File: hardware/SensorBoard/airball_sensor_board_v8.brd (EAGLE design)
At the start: 5.6 x 9.2 mm, 61 parts, among them IC1 CP2102, J2 USB Female Type C Connector, T1 BC846, T2 BC846, U1 BQ24075, U2 BQ27441-G1, U3 BMP388, U4 ESP-WROOM-32, U7 SP0503BAHT

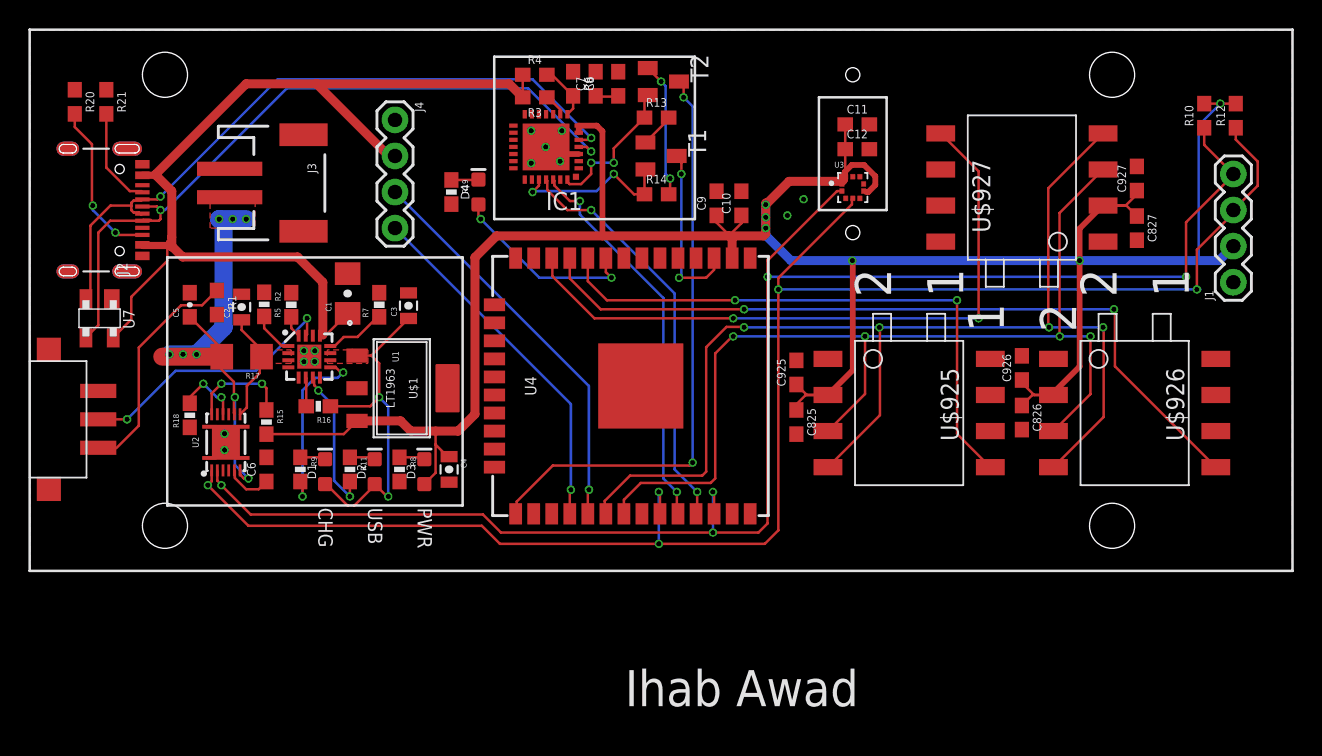
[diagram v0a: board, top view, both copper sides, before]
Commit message: Finishing touches to the board, sent to manufacturing.
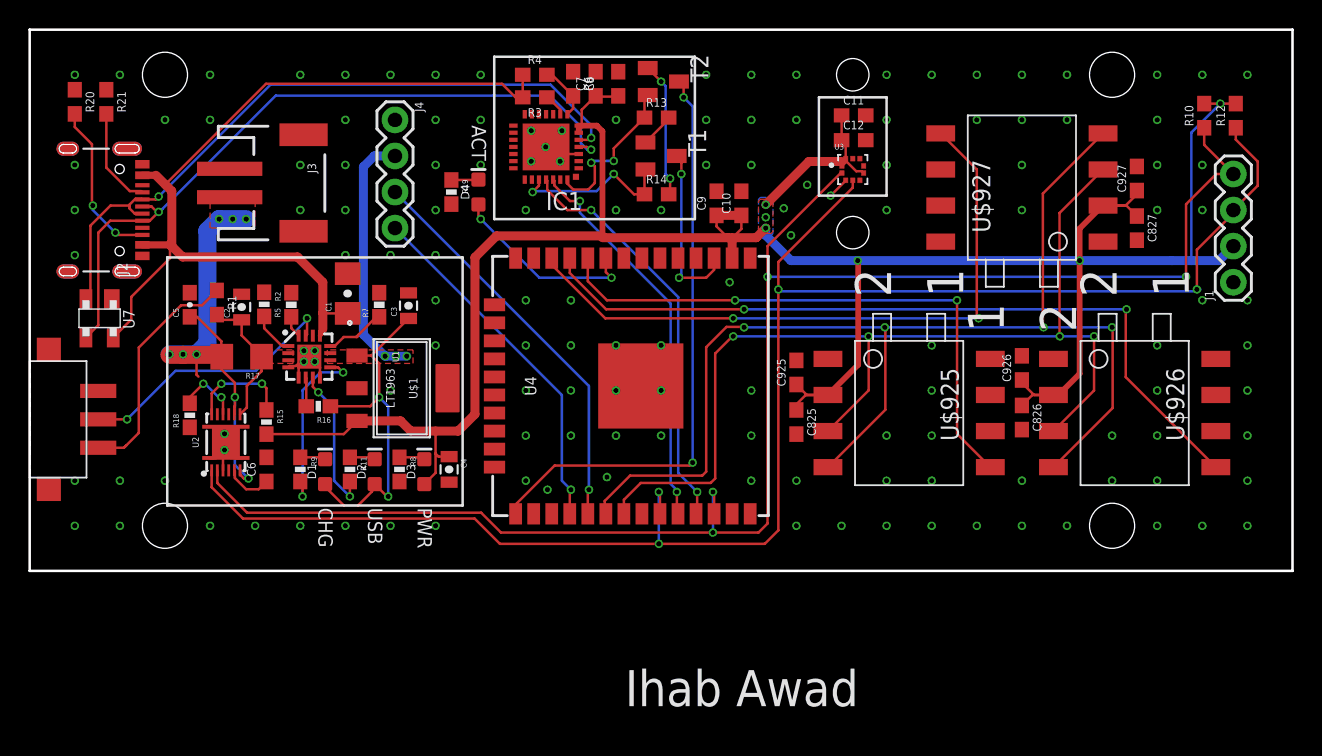
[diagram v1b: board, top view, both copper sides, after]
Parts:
- moved U3 1.27 mm to (57.9, 28.3)
- moved C11 0.68 mm to (58.0, 32.1)
- moved C12 0.68 mm to (58.0, 30.3)
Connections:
- net V_SUPPLY_UNREG: now also J4.2
- net V_USB: no longer J4.2
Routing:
- net V_SUPPLY_UNREG: track 25.6 -> 44.3 mm, vias 2 -> 5
- net GND: track 2.54 -> 17.1 mm, vias 3 -> 139
- net V_USB: track 72.9 -> 64.2 mm
- net V_BATT: track 7.97 -> 9.87 mm
- net SCL: track 113.9 -> 115.7 mm, vias 5 -> 4
- net BATTERY_IN: track 33.4 -> 35.0 mm
- net SYSOFF_OFF: track 14.9 -> 16.5 mm
- net SCLK: track 84.1 -> 85.4 mm
- net SDA: track 117.8 -> 118.9 mm, vias 5 -> 4
- net USB_DTR: track 10.3 -> 11.4 mm
- net USB_D+: track 51.9 -> 51.0 mm
- added copper zone on layer 1, net VCC
- added copper zone on layer 16, net VCC
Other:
- board size 5.6 x 9.2 mm -> 88.9 x 38.1 mm
- board text added: "ACT"
